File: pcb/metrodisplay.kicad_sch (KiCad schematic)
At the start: 23 parts, among them J1 USB_C_Receptacle_PowerOnly_6P, J2 Conn_02x08_Counter_Clockwise, J3 Screw_Terminal_01x02, SW1 SW_Push, U1 ESP32-DEVKITC

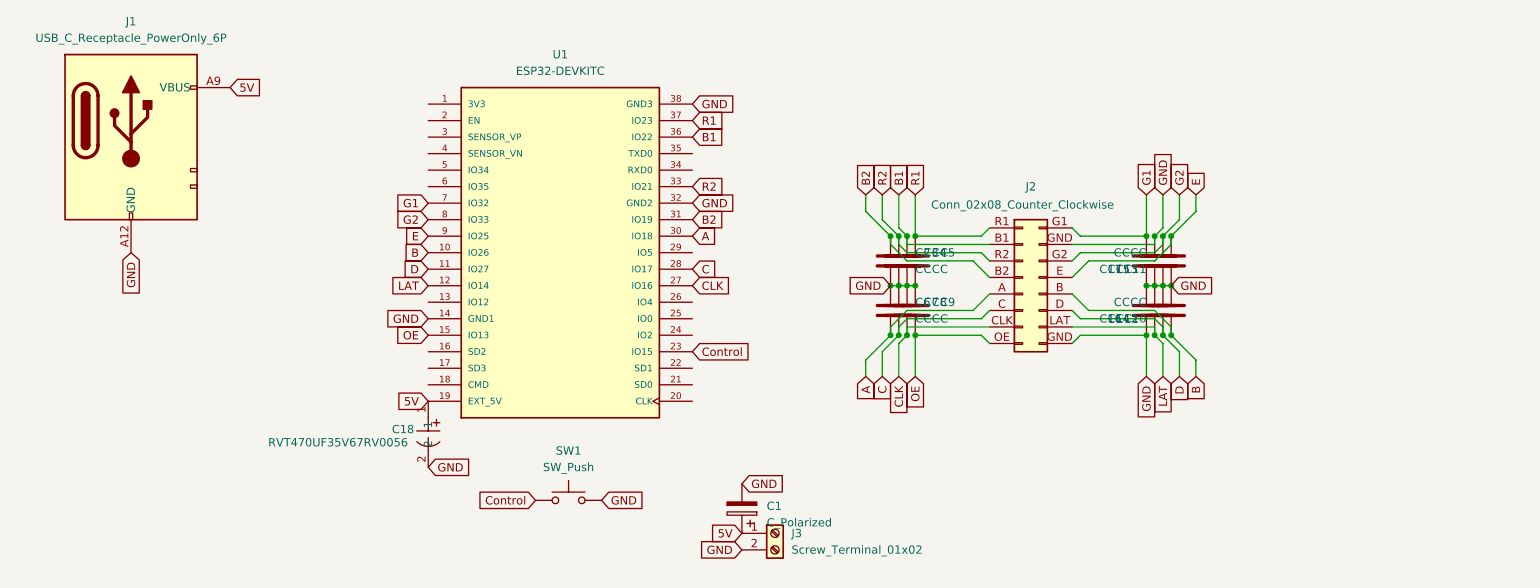
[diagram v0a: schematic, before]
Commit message: PCB Routing test
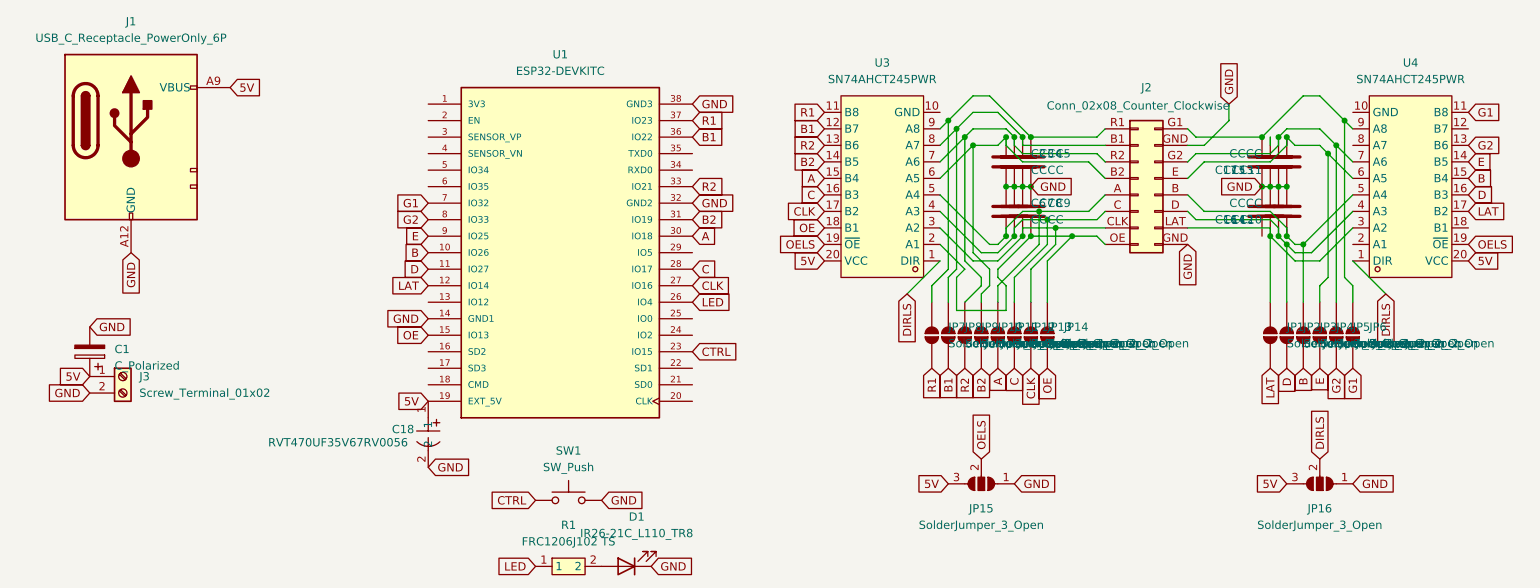
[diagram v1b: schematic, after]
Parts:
- added D1: IR26-21C_L110_TR8, LED_SMD:LED_1206_3216Metric, symbol LED:IR26-21C_L110_TR8
- added JP1, JP10, JP11, JP12, JP13, JP14, JP2, JP3, JP4, JP5, JP6, JP7, JP8, JP9: SolderJumper_2_Open, Jumper:SolderJumper-2_P1.3mm_Open_TrianglePad1.0x1.5mm, symbol Jumper:SolderJumper_2_Open
- added JP15, JP16: SolderJumper_3_Open, Jumper:SolderJumper-3_P2.0mm_Open_TrianglePad1.0x1.5mm, symbol Jumper:SolderJumper_3_Open
- added R1: FRC1206J102 TS, easyeda2kicad:R1206, symbol easyeda2kicad:FRC1206J102TS
- added U3, U4: SN74AHCT245PWR, easyeda2kicad:TSSOP-20_L6.5-W4.4-P0.65-LS6.4-BL, symbol easyeda2kicad:SN74AHCT245PWR
- C10, C11, C12, C13, C14, C15, C16, C17, C2, C3, C4, C5, C6, C7, C8, C9: footprint (none) -> easyeda2kicad:C1206
- J2: footprint Connector_PinHeader_2.54mm:PinHeader_2x08_P2.54mm_Vertical -> easyeda2kicad:PinHeader_2x08_P2.54mm_Vertical_MD
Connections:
- net 5V: now also JP15.3 (B), JP16.3 (B), U3.20 (VCC), U4.20 (VCC)
- net A: now also JP11.1 (A), U3.15 (B4); no longer C6.2, J2.A (Pin_5)
- net B: now also JP3.1 (A), U4.15 (B4); no longer C10.1, J2.B (Pin_12)
- net B1: now also JP8.1 (A), U3.12 (B7); no longer C4.1, J2.B1 (Pin_2)
- net B2: now also JP10.1 (A), U3.14 (B5); no longer C2.1, J2.B2 (Pin_4)
- net C: now also JP12.1 (A), U3.16 (B3); no longer C7.2, J2.C (Pin_6)
- net CLK: now also JP13.1 (A), U3.17 (B2); no longer C8.2, J2.CLK (Pin_7)
- net D: now also JP2.1 (A), U4.16 (B3); no longer C12.1, J2.D (Pin_11)
- net E: now also JP4.1 (A), U4.14 (B5); no longer C11.2, J2.E (Pin_13)
- net G1: now also JP6.1 (A), U4.11 (B8); no longer C17.2, J2.G1 (Pin_16)
- net G2: now also JP5.1 (A), U4.13 (B6); no longer C13.2, J2.G2 (Pin_14)
- net GND: now also D1.1 (K), JP15.1 (A), JP16.1 (A); no longer C15.2, C16.1
- net LAT: now also JP1.1 (A), U4.17 (B2); no longer C14.1, J2.LAT (Pin_10)
- net OE: now also JP14.1 (A), U3.18 (B1); no longer C9.2, J2.OE (Pin_8)
- net R1: now also JP7.1 (A), U3.11 (B8); no longer C5.1, J2.R1 (Pin_1)
- net R2: now also JP9.1 (A), U3.13 (B6); no longer C3.1, J2.R2 (Pin_3)
- net LED: now reaches U1.26 (IO4)
- net LED: now also R1.1
- net Control renamed CTRL
- new net: D1.2 (A), R1.2
- new net: C3.1, J2.R2 (Pin_3), JP9.2 (B), U3.7 (A6)
- new net: C8.2, J2.CLK (Pin_7), JP13.2 (B), U3.3 (A2)
- new net: C14.1, J2.LAT (Pin_10), JP1.2 (B), U4.3 (A2)
- new net: C12.1, J2.D (Pin_11), JP2.2 (B), U4.4 (A3)
- new net: C10.1, J2.B (Pin_12), JP3.2 (B), U4.5 (A4)
- new net: C11.2, J2.E (Pin_13), JP4.2 (B), U4.6 (A5)
- new net: C13.2, J2.G2 (Pin_14), JP5.2 (B), U4.7 (A6)
- new net: C17.2, J2.G1 (Pin_16), JP6.2 (B), U4.9 (A8)
- new net: C5.1, J2.R1 (Pin_1), JP7.2 (B), U3.9 (A8)
- new net: C9.2, J2.OE (Pin_8), JP14.2 (B), U3.2 (A1)
- new net: C7.2, J2.C (Pin_6), JP12.2 (B), U3.4 (A3)
- new net: C6.2, J2.A (Pin_5), JP11.2 (B), U3.5 (A4)
- new net: C2.1, J2.B2 (Pin_4), JP10.2 (B), U3.6 (A5)
- new net: C4.1, J2.B1 (Pin_2), JP8.2 (B), U3.8 (A7)
- new net DIRLS: JP16.2 (C), U3.1 (DIR), U4.1 (DIR)
- new net OELS: JP15.2 (C), U3.19 (~{OE}), U4.19 (~{OE})
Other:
- moved on the sheet: C1, C10, C11, C12, C13, C14, C15, C16, C17, C2, C3, C4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

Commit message: PCB routing done
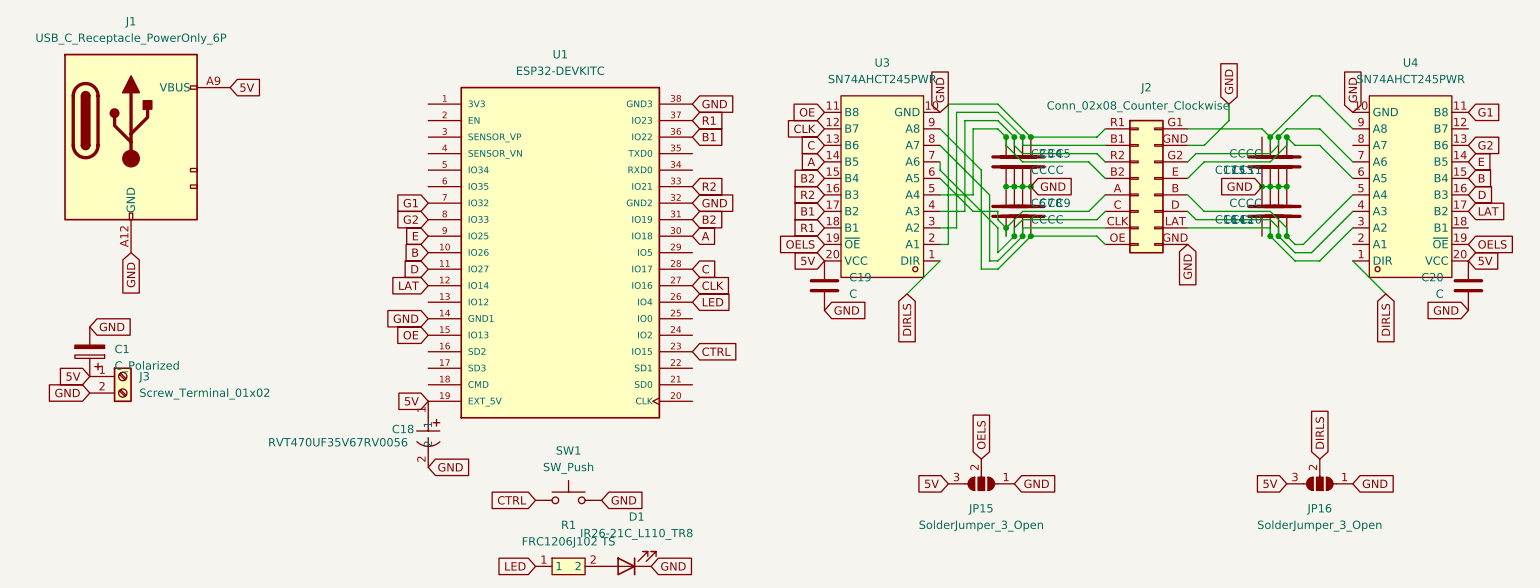
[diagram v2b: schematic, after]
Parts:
- removed JP1, JP10, JP11, JP12, JP13, JP14, JP2, JP3, JP4, JP5, JP6, JP7, JP8, JP9: SolderJumper_2_Open, Jumper:SolderJumper-2_P1.3mm_Open_TrianglePad1.0x1.5mm, symbol Jumper:SolderJumper_2_Open
- added C19, C20: C, easyeda2kicad:C1206, symbol Device:C
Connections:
- net 5V: now also C19.1, C20.1
- net A: now also U3.14 (B5); no longer U3.15 (B4)
- net B1: now also U3.17 (B2); no longer U3.12 (B7)
- net B2: now also U3.15 (B4); no longer U3.14 (B5)
- net C: now also U3.13 (B6); no longer U3.16 (B3)
- net CLK: now also U3.12 (B7); no longer U3.17 (B2)
- net GND: now also U3.10 (GND), U4.10 (GND), C19.2, C20.2
- net OE: now also U3.11 (B8); no longer U3.18 (B1)
- net R1: now also U3.18 (B1); no longer U3.11 (B8)
- net R2: now also U3.16 (B3); no longer U3.13 (B6)
- net at C3.1, J2.R2 (Pin_3): now also U3.4 (A3); no longer U3.7 (A6)
- net at C8.2, J2.CLK (Pin_7): now also U3.8 (A7); no longer U3.3 (A2)
- net at J2.G1 (Pin_16), U4.9 (A8): now also C15.2; no longer C17.2
- net at C5.1, J2.R1 (Pin_1): now also U3.2 (A1); no longer U3.9 (A8)
- net at C9.2, J2.OE (Pin_8): now also U3.9 (A8); no longer U3.2 (A1)
- net at C7.2, J2.C (Pin_6): now also U3.7 (A6); no longer U3.4 (A3)
- net at C6.2, J2.A (Pin_5): now also U3.6 (A5); no longer U3.5 (A4)
- net at C2.1, J2.B2 (Pin_4): now also U3.5 (A4); no longer U3.6 (A5)
- net at C4.1, J2.B1 (Pin_2): now also U3.3 (A2); no longer U3.8 (A7)
